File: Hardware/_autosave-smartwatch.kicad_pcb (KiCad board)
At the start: 4 copper layers, 36.5 x 38 mm, 50 parts, among them IC1 W25Q256JVEIQ, IC2 NORA-B120-00B, IC3 LM66200DRLR, J3 DF37NB-24DS-0.4V51, U1 MAX17048G+T10, U11 MCP73831T-2ACI/OT, U2 TPD2EUSB30DRTR, U3 MAX30102, U4 TPS63031DSK, U5 CAM-M8C-0, U6 AP7313-18SAG-7, U7 BMI270, U8 LIS2MDLTR, U9 TPD2EUSB30DRTR, X2 9HT10-32.768KBZC-T

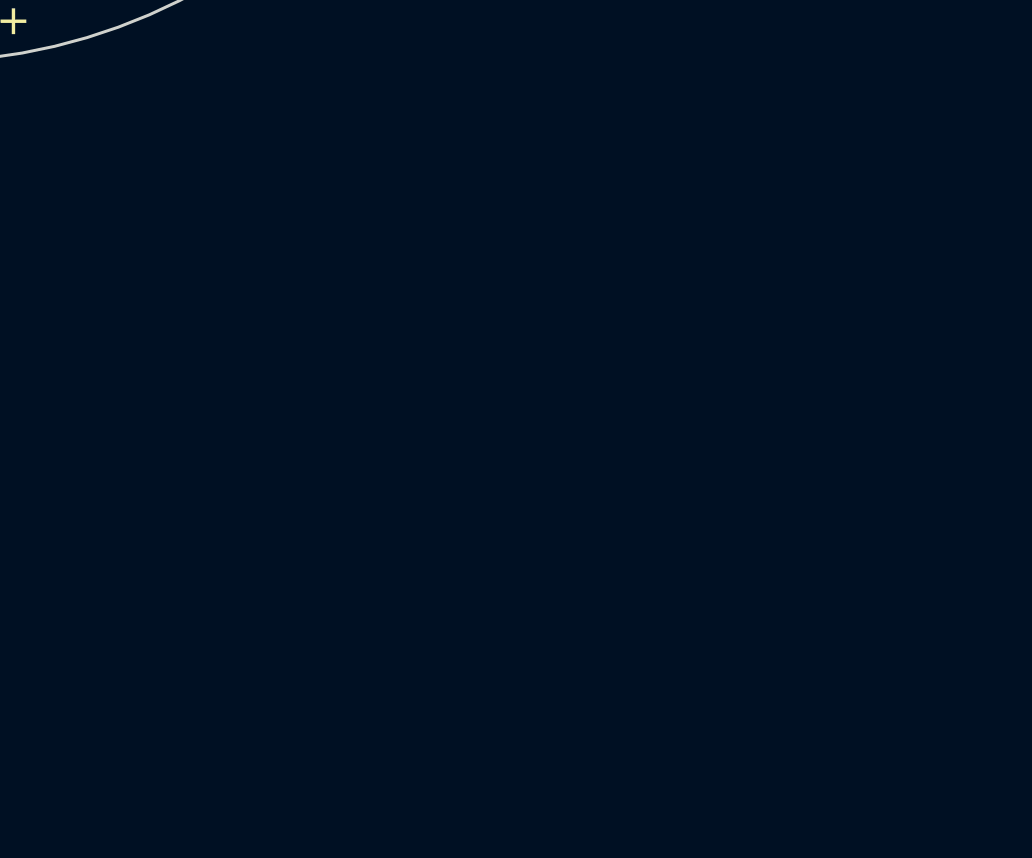
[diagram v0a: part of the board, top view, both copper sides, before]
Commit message: v3 schema complete
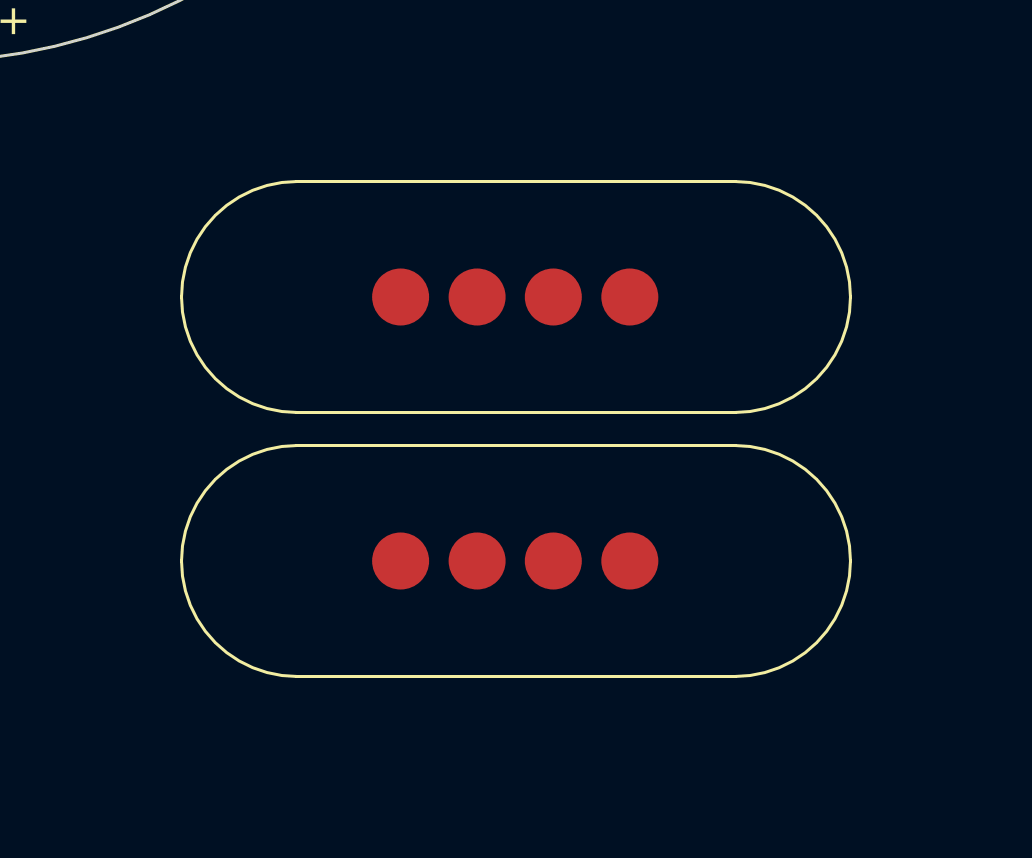
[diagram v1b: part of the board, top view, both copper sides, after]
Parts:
- added J1: Conn_01x04, Pogo_Female_4pin:Pogo_Female_4Pin, F.Cu at (164.7, 124.6)
- added J2: Conn_01x04, Pogo_Female_4pin:Pogo_Female_4Pin, F.Cu at (164.7, 133.4)
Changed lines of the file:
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@@
+    )
+  )
+  (footprint "Pogo_Female_4pin:Pogo_Female_4Pin" (layer "F.Cu")
+    (at 164.656 124.57)
+    (descr "Capacitor SMD 0402 (1005 Metric), square (rectangular) end terminal, IPC_7351 nominal, (Body size source: IPC-SM-782 page 76, https://www.pcb-3d.com/wordpress/wp-content/uploads/ipc-sm-782a_amendment_1_and_2.pdf), generated with kicad-footprint-generator")
+    (tags "capacitor")
+    (property "Sheetfile" "smartwatch.kicad_sch")
+    (property "Sheetname" "")
+    (property "ki_description" "Generic connector, single row, 01x04, script generated (kicad-library-utils/schlib/autogen/connector/)")
+    (property "ki_keywords" "connector")
+    (attr smd)
+    (fp_text reference "J1" (at 4.318 -2.4892) (layer "F.SilkS") hide
+        (effects (font (size 1 1) (thickness 0.15)))
+    )
+    (fp_text value "Conn_01x04" (at 4.468 2.3108) (layer "F.Fab") hide
+        (effects (font (size 1 1) (thickness 0.15)))
+    )
+    (fp_line (start -3.21 3.85) (end 11.39 3.85)
+      (stroke (width 0.1) (type default)) (layer "F.SilkS"))
+    (fp_line (start 11.39 -3.85) (end -3.21 -3.85)
+      (stroke (width 0.1) (type default)) (layer "F.SilkS"))
+    (fp_arc (start -7.06 0) (mid -5.932361 -2.722361) (end -3.21 -3.85)
+      (stroke (width 0.1) (type default)) (layer "F.SilkS"))
+    (fp_arc (start -3.21 3.85) (mid -5.932361 2.722361) (end -7.06 0)
+      (stroke (width 0.1) (type default)) (layer "F.SilkS"))
+    (fp_arc (start 11.39 -3.85) (mid 14.112361 -2.722361) (end 15.24 0)
+      (stroke (width 0.1) (type default)) (layer "F.SilkS"))
+    (fp_arc (start 15.24 0) (mid 14.112361 2.722361) (end 11.39 3.85)
+      (stroke (width 0.1) (type default)) (layer "F.SilkS"))
+    (pad "1" smd circle (at 0.244 0) (size 1.9 1.9) (layers "F.Cu" "F.Paste" "F.Mask")
+      (net 43 "VIN_SWD") (pinfunction "Pin_1") (pintype "passive"))
+    (pad "2" smd circle (at 2.794 0) (size 1.9 1.9) (layers "F.Cu" "F.Paste" "F.Mask")
+      (net 110 "/USB_N") (pinfunction "Pin_2") (pintype "passive"))
+    (pad "3" smd circle (at 5.334 0) (size 1.9 1.9) (layers "F.Cu" "F.Paste" "F.Mask")
+      (net 104 "/USB_P") (pinfunction "Pin_3") (pintype "passive"))
+    (pad "4" smd circle (at 7.884 0) (size 1.9 1.9) (layers "F.Cu" "F.Paste" "F.Mask")
+      (net 1 "GND") (pinfunction "Pin_4") (pintype "passive"))
+    (model "${KICAD6_3DMODEL_DIR}/Capacitor_SMD.3dshapes/C_0402_1005Metric.wrl"
+      (offset (xyz 0 0 0))
+      (scale (xyz 1 1 1))
+      (rotate (xyz 0 0 0))
     )
   )
@@
       (offset (xyz 0 0 0))
       (scale (xyz 1 1 1))
+      (rotate (xyz 0 0 0))
+    )
+  )
+  (footprint "Pogo_Female_4pin:Pogo_Female_4Pin" (layer "F.Cu")
+    (at 164.656 133.37)
+    (descr "Capacitor SMD 0402 (1005 Metric), square (rectangular) end terminal, IPC_7351 nominal, (Body size source: IPC-SM-782 page 76, https://www.pcb-3d.com/wordpress/wp-content/uploads/ipc-sm-782a_amendment_1_and_2.pdf), generated with kicad-footprint-generator")
+    (tags "capacitor")
+    (property "Sheetfile" "smartwatch.kicad_sch")
+    (property "Sheetname" "")
+    (property "ki_description" "Generic connector, single row, 01x04, script generated (kicad-library-utils/schlib/autogen/connector/)")
+    (property "ki_keywords" "connector")
+    (attr smd)
+    (fp_text reference "J2" (at 4.318 -2.4892) (layer "F.SilkS") hide
+        (effects (font (size 1 1) (thickness 0.15)))
+    )
+    (fp_text value "Conn_01x04" (at 4.468 2.3108) (layer "F.Fab") hide
+        (effects (font (size 1 1) (thickness 0.15)))
+    )
+    (fp_line (start -3.21 3.85) (end 11.39 3.85)
+      (stroke (width 0.1) (type default)) (layer "F.SilkS"))
+    (fp_line (start 11.39 -3.85) (end -3.21 -3.85)
+      (stroke (width 0.1) (type default)) (layer "F.SilkS"))
+    (fp_arc (start -7.06 0) (mid -5.932361 -2.722361) (end -3.21 -3.85)
+      (stroke (width 0.1) (type default)) (layer "F.SilkS"))
+    (fp_arc (start -3.21 3.85) (mid -5.932361 2.722361) (end -7.06 0)
+      (stroke (width 0.1) (type default)) (layer "F.SilkS"))
+    (fp_arc (start 11.39 -3.85) (mid 14.112361 -2.722361) (end 15.24 0)
+      (stroke (width 0.1) (type default)) (layer "F.SilkS"))
+    (fp_arc (start 15.24 0) (mid 14.112361 2.722361) (end 11.39 3.85)
+      (stroke (width 0.1) (type default)) (layer "F.SilkS"))
+    (pad "1" smd circle (at 0.244 0) (size 1.9 1.9) (layers "F.Cu" "F.Paste" "F.Mask")
+      (net 43 "VIN_SWD") (pinfunction "Pin_1") (pintype "passive"))
+    (pad "2" smd circle (at 2.794 0) (size 1.9 1.9) (layers "F.Cu" "F.Paste" "F.Mask")
+      (net 61 "/SWDIO") (pinfunction "Pin_2") (pintype "passive"))
+    (pad "3" smd circle (at 5.334 0) (size 1.9 1.9) (layers "F.Cu" "F.Paste" "F.Mask")
+      (net 64 "/SWDCLK") (pinfunction "Pin_3") (pintype "passive"))
+    (pad "4" smd circle (at 7.884 0) (size 1.9 1.9) (layers "F.Cu" "F.Paste" "F.Mask")
+      (net 1 "GND") (pinfunction "Pin_4") (pintype "passive"))
+    (model "${KICAD6_3DMODEL_DIR}/Capacitor_SMD.3dshapes/C_0402_1005Metric.wrl"
+      (offset (xyz 0 0 0))
+      (scale (xyz 1 1 1))
